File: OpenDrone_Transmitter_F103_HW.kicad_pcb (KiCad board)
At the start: 2 copper layers, 52 x 32 mm, 75 parts, among them J1 Conn_01x03, J10 Conn_01x04, J11 Conn_01x03, J12 Conn_01x04, J13 Conn_01x02, J14 Conn_01x05, J15 Conn_01x02, J16 Conn_02x04_Odd_Even, J17 Conn_01x02, J18 Conn_01x02, J19 Conn_01x03, J2 Conn_01x05, J20 Conn_01x02, J21 Conn_01x02, J22 Conn_01x02, J3 Conn_01x03, J4 Conn_01x03, J5 Conn_01x03, J6 Conn_01x02, J7 Conn_01x02, J8 Conn_01x03, J9 Conn_01x03, SW1 RESET, U1 STM32F103C8Tx, U2 AMS1117-3.3, U3 TPS54331, Y2 Crystal_GND24

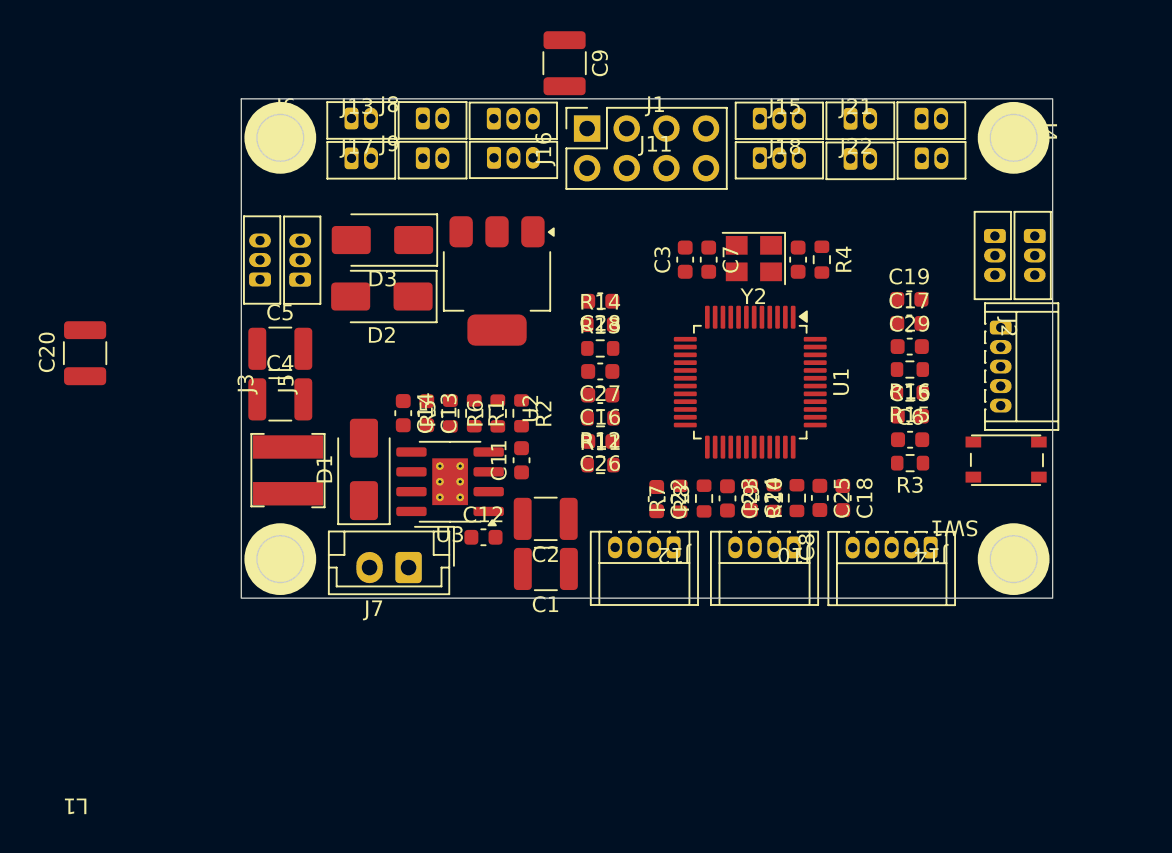
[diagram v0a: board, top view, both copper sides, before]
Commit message: update project
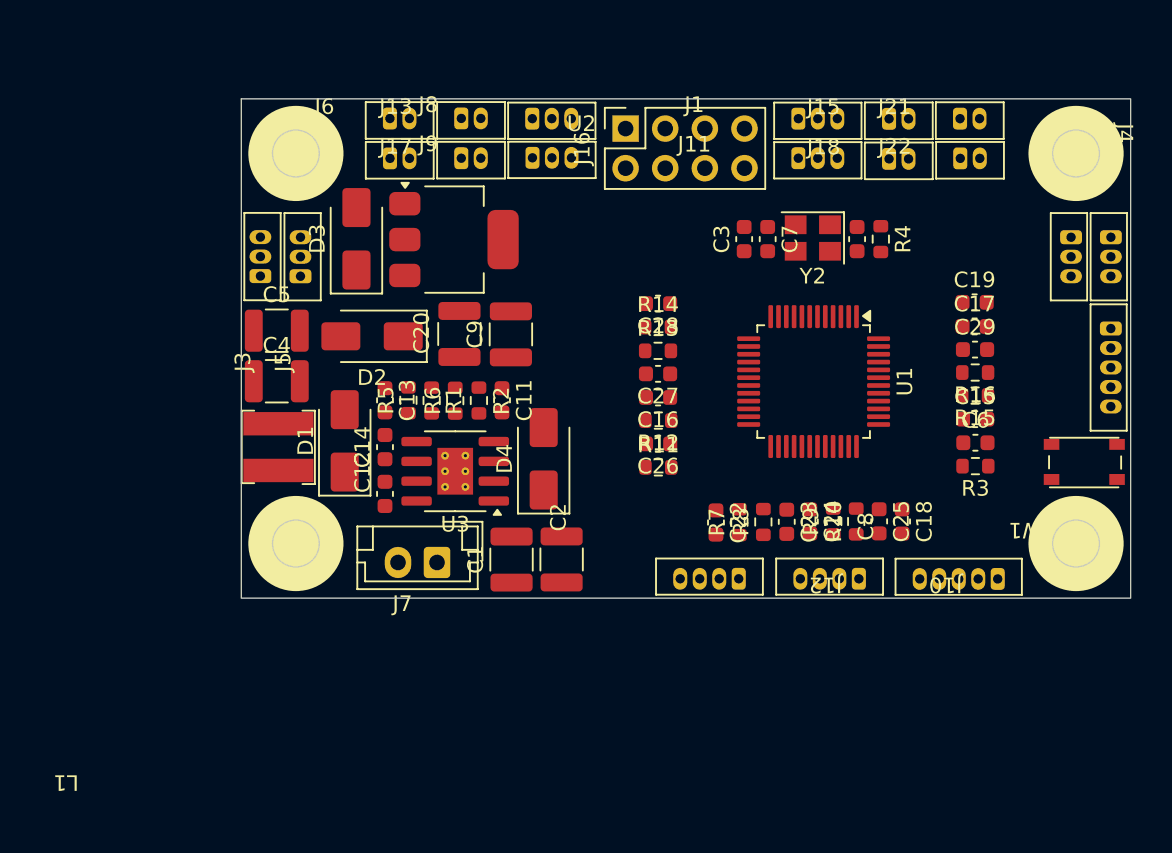
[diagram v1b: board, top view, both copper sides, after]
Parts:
- added D4: SS24, Diode_SMD:D_SMA, F.Cu at (182.9, 100.2)
- J10, J12: footprint Footprint:Connector_XH_1x04_P1.25mm_Horizontal -> Footprint:Connector_XH_1x04_P1.25mm_Vertical
- J14, J2: footprint Footprint:Connector_XH_1x05_P1.25mm_Horizontal -> Footprint:Connector_XH_1x05_P1.25mm_Vertical
- moved C20 24.0 mm to (177.6, 92.2)
- moved C9 17.7 mm to (180.8, 92.2), turned to 90 degrees
- moved J2 7.06 mm to (219.3, 91.8)
- moved C12 6.90 mm to (172.8, 102.5), turned to 90 degrees
- moved SW1 5.01 mm to (217.6, 100.4)
- moved J19 4.88 mm to (216.8, 86.0)
- moved J4 4.88 mm to (219.3, 86.0)
- moved J14 4.74 mm to (212.1, 107.9)
- moved J10 4.63 mm to (203.2, 107.9)
- moved J12 4.63 mm to (195.4, 107.9)
- moved C17 4.19 mm to (210.6, 91.7)
- moved C29 4.19 mm to (210.6, 93.2)
- moved R15 4.19 mm to (210.6, 96.2)
- moved C15 4.19 mm to (210.6, 97.7)
- moved C19 4.19 mm to (210.6, 90.2)
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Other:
- board size 52 x 32 mm -> 57 x 32 mm
